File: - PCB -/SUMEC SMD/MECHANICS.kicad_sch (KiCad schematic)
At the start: 9 parts, among them J1 Conn_01x01_Pin, SW1 SW_SPDT, SW3 SW_Push

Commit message: PCB Schematic SMD
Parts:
- SW3: footprint Button_Switch_THT:SW_PUSH_6mm -> Button_Switch_SMD:SW_SPST_B3U-1000P
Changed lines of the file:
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@@
       (effects (font (size 1.27 1.27)))
     )
-    (property "Footprint" "Button_Switch_THT:SW_PUSH_6mm" (at 92.71 125.73 0)
+    (property "Footprint" "Button_Switch_SMD:SW_SPST_B3U-1000P" (at 92.71 125.73 0)
       (effects (font (size 1.27 1.27)) hide)
     )

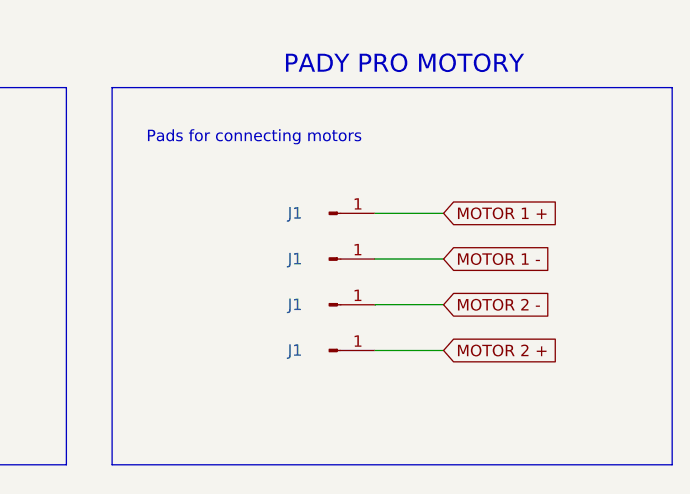
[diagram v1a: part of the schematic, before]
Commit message: PCB SMD update
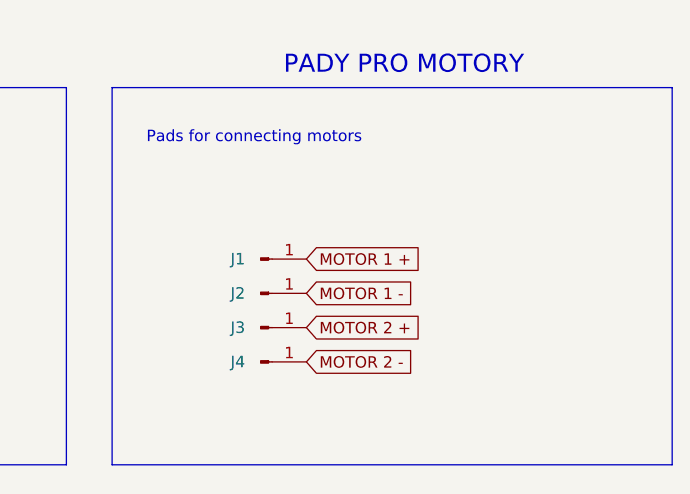
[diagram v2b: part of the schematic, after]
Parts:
- removed J1 (x4): Conn_01x01_Pin, Connector_Wire:SolderWire-0.5sqmm_1x01_D0.9mm_OD2.3mm, symbol Connector:Conn_01x01_Pin
- added J1, J2, J3, J4: Conn_01x01_Pin, Connector_Wire:SolderWire-0.5sqmm_1x01_D0.9mm_OD2.1mm, symbol Connector:Conn_01x01_Pin
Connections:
- net MOTOR 1 +: now also J1.1 (Pin_1)
- net MOTOR 1 -: now also J2.1 (Pin_1)
- net MOTOR 2 +: now also J3.1 (Pin_1)
- net MOTOR 2 -: now also J4.1 (Pin_1)

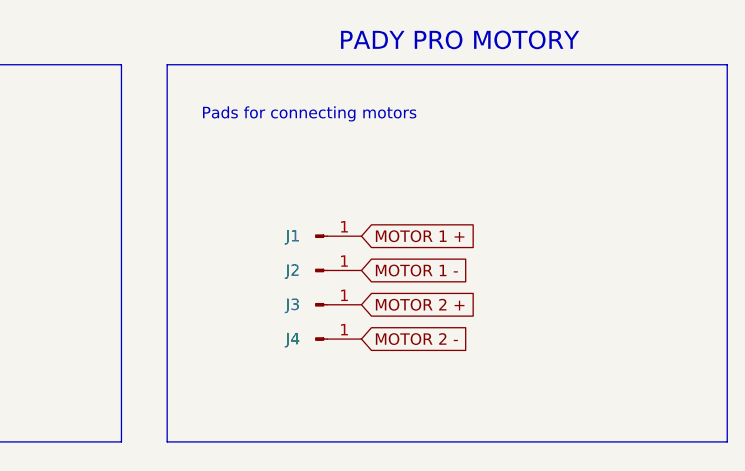
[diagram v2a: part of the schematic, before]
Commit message: PCB smd - schematic update
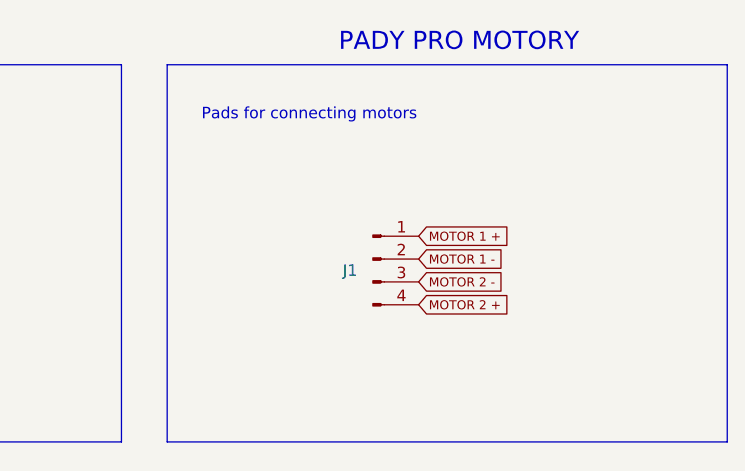
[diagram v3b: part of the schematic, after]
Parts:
- removed J1, J2, J3, J4: Conn_01x01_Pin, Connector_Wire:SolderWire-0.5sqmm_1x01_D0.9mm_OD2.1mm, symbol Connector:Conn_01x01_Pin
- added J1: Conn_01x04_Pin, Connector_PinHeader_2.54mm:PinHeader_1x04_P2.54mm_Vertical, symbol Connector:Conn_01x04_Pin
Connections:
- net MOTOR 1 +: now also J1.1 (Pin_1)
- net MOTOR 1 -: now also J1.2 (Pin_2)
- net MOTOR 2 +: now also J1.4 (Pin_4)
- net MOTOR 2 -: now also J1.3 (Pin_3)
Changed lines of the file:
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@@
     (effects (font (size 1.27 1.27) italic) (justify left bottom))
   )
-  (global_label "MOTOR 1 +" (shape input) (at 170.18 118.11 0) (fields_autoplaced)
-    (effects (font (size 1.27 1.27)) (justify left))
-    (property "Intersheetrefs" "${INTERSHEET_REFS}" (at 184.1529 118.11 0)
-      (effects (font (size 1.27 1.27)) (justify left) hide)
-    )
-  )
-  (global_label "MOTOR 2 +" (shape input) (at 170.18 125.73 0) (fields_autoplaced)
-    (effects (font (size 1.27 1.27)) (justify left))
-    (property "Intersheetrefs" "${INTERSHEET_REFS}" (at 184.1529 125.73 0)
-      (effects (font (size 1.27 1.27)) (justify left) hide)
-    )
-  )
-  (global_label "MOTOR 2 -" (shape input) (at 170.18 129.54 0) (fields_autoplaced)
-    (effects (font (size 1.27 1.27)) (justify left))
-    (property "Intersheetrefs" "${INTERSHEET_REFS}" (at 184.1529 129.54 0)
-      (effects (font (size 1.27 1.27)) (justify left) hide)
-    )
-  )
-  (global_label "MOTOR 1 -" (shape input) (at 170.18 121.92 0) (fields_autoplaced)
-    (effects (font (size 1.27 1.27)) (justify left))
-    (property "Intersheetrefs" "${INTERSHEET_REFS}" (at 184.1529 121.92 0)
+  (global_label "MOTOR 1 +" (shape input) (at 176.53 118.11 0) (fields_autoplaced)
+    (effects (font (size 1 1)) (justify left))
+    (property "Intersheetrefs" "${INTERSHEET_REFS}" (at 187.5322 118.11 0)
+      (effects (font (size 1.27 1.27)) (justify left) hide)
+    )
+  )
+  (global_label "MOTOR 2 +" (shape input) (at 176.53 125.73 0) (fields_autoplaced)
+    (effects (font (size 1 1)) (justify left))
+    (property "Intersheetrefs" "${INTERSHEET_REFS}" (at 187.5322 125.73 0)
+      (effects (font (size 1.27 1.27)) (justify left) hide)
+    )
+  )
+  (global_label "MOTOR 2 -" (shape input) (at 176.53 123.19 0) (fields_autoplaced)
+    (effects (font (size 1 1)) (justify left))
+    (property "Intersheetrefs" "${INTERSHEET_REFS}" (at 187.5322 123.19 0)
+      (effects (font (size 1.27 1.27)) (justify left) hide)
+    )
+  )
+  (global_label "MOTOR 1 -" (shape input) (at 176.53 120.65 0) (fields_autoplaced)
+    (effects (font (size 1 1)) (justify left))
+    (property "Intersheetrefs" "${INTERSHEET_REFS}" (at 187.5322 120.65 0)
       (effects (font (size 1.27 1.27)) (justify left) hide)
     )
@@
     )
   )
-  (symbol (lib_id "Connector:Conn_01x01_Pin") (at 165.1 121.92 0) (unit 1)
-    (in_bom yes) (on_board yes) (dnp no)
-    (property "Reference" "J2" (at 162.56 121.92 0)
-      (effects (font (size 1.27 1.27)))
-    )
-    (property "Value" "Conn_01x01_Pin" (at 165.735 120.65 0)
-      (effects (font (size 1.27 1.27)) hide)
-    )
-    (property "Footprint" "Connector_Wire:SolderWire-0.5sqmm_1x01_D0.9mm_OD2.1mm" (at 165.1 121.92 0)
-      (effects (font (size 1.27 1.27)) hide)
-    )
-    (property "Datasheet" "~" (at 165.1 121.92 0)
-      (effects (font (size 1.27 1.27)) hide)
-    )
-    (pin "1")
-    (instances
-      (project "sumec"
-        (path "/fc70a1a8-ed7c-4a0f-9b1a-f23293528385/05a35bad-c108-46ad-8f95-76319a60a14f"
-          (reference "J2") (unit 1)
-        )
-      )
-    )
-  )
   (symbol (lib_id "Mechanical:MountingHole") (at 72.39 68.58 0) (unit 1)
     (in_bom yes) (on_board yes) (dnp no) (fields_autoplaced)
@@
     )
   )
+  (symbol (lib_id "Connector:Conn_01x04_Pin") (at 171.45 120.65 0) (unit 1)
+    (in_bom yes) (on_board yes) (dnp no)
+    (property "Reference" "J1" (at 168.91 121.92 0)
+      (effects (font (size 1.27 1.27)))
+    )
+    (property "Value" "Conn_01x04_Pin" (at 172.085 116.84 0)
+      (effects (font (size 1.27 1.27)) hide)
+    )
+    (property "Footprint" "Connector_PinHeader_2.54mm:PinHeader_1x04_P2.54mm_Vertical" (at 171.45 120.65 0)
+      (effects (font (size 1.27 1.27)) hide)
+    )
+    (property "Datasheet" "~" (at 171.45 120.65 0)
+      (effects (font (size 1.27 1.27)) hide)
+    )
+    (pin "1")
+    (pin "2")
+    (pin "3")
+    (pin "4")
+    (instances
+      (project "sumec"
+        (path "/fc70a1a8-ed7c-4a0f-9b1a-f23293528385/05a35bad-c108-46ad-8f95-76319a60a14f"
+          (reference "J1") (unit 1)
+        )
+      )
+    )
+  )
   (symbol (lib_id "power:+3V3") (at 86.36 130.81 90) (unit 1)
     (in_bom yes) (on_board yes) (dnp no) (fields_autoplaced)
@@
         (path "/fc70a1a8-ed7c-4a0f-9b1a-f23293528385/05a35bad-c108-46ad-8f95-76319a60a14f"
           (reference "#PWR02") (unit 1)
-        )
-      )
-    )
-  )
-  (symbol (lib_id "Connector:Conn_01x01_Pin") (at 165.1 125.73 0) (unit 1)
-    (in_bom yes) (on_board yes) (dnp no)
-    (property "Reference" "J3" (at 162.56 125.73 0)
-      (effects (font (size 1.27 1.27)))
-    )
-    (property "Value" "Conn_01x01_Pin" (at 165.735 124.46 0)
-      (effects (font (size 1.27 1.27)) hide)
-    )
-    (property "Footprint" "Connector_Wire:SolderWire-0.5sqmm_1x01_D0.9mm_OD2.1mm" (at 165.1 125.73 0)
-      (effects (font (size 1.27 1.27)) hide)
-    )
-    (property "Datasheet" "~" (at 165.1 125.73 0)
-      (effects (font (size 1.27 1.27)) hide)
-    )
-    (pin "1")
-    (instances
-      (project "sumec"
-        (path "/fc70a1a8-ed7c-4a0f-9b1a-f23293528385/05a35bad-c108-46ad-8f95-76319a60a14f"
-          (reference "J3") (unit 1)
         )
       )
@@
         (path "/fc70a1a8-ed7c-4a0f-9b1a-f23293528385/05a35bad-c108-46ad-8f95-76319a60a14f"
           (reference "H1") (unit 1)
-        )
-      )
-    )
-  )
-  (symbol (lib_id "Connector:Conn_01x01_Pin") (at 165.1 118.11 0) (unit 1)
-    (in_bom yes) (on_board yes) (dnp no)
-    (property "Reference" "J1" (at 162.56 118.11 0)
-      (effects (font (size 1.27 1.27)))
-    )
-    (property "Value" "Conn_01x01_Pin" (at 165.735 116.84 0)
-      (effects (font (size 1.27 1.27)) hide)
-    )
-    (property "Footprint" "Connector_Wire:SolderWire-0.5sqmm_1x01_D0.9mm_OD2.1mm" (at 165.1 118.11 0)
-      (effects (font (size 1.27 1.27)) hide)
-    )
-    (property "Datasheet" "~" (at 165.1 118.11 0)
-      (effects (font (size 1.27 1.27)) hide)
-    )
-    (pin "1")
-    (instances
-      (project "sumec"
-        (path "/fc70a1a8-ed7c-4a0f-9b1a-f23293528385/05a35bad-c108-46ad-8f95-76319a60a14f"
-          (reference "J1") (unit 1)
         )
       )
@@
         )
       )
-    )
-  )
-  (symbol (lib_id "Connector:Conn_01x01_Pin") (at 165.1 129.54 0) (unit 1)
-    (in_bom yes) (on_board yes) (dnp no)
-    (property "Reference" "J4" (at 162.56 129.54 0)
-      (effects (font (size 1.27 1.27)))
-    )
-    (property "Value" "Conn_01x01_Pin" (at 165.735 128.27 0)
-      (effects (font (size 1.27 1.27)) hide)
-    )
-    (property "Footprint" "Connector_Wire:SolderWire-0.5sqmm_1x01_D0.9mm_OD2.1mm" (at 165.1 129.54 0)
-      (effects (font (size 1.27 1.27)) hide)
-    )
-    (property "Datasheet" "~" (at 165.1 129.54 0)
-      (effects (font (size 1.27 1.27)) hide)
-    )
-    (pin "1")
-    (instances
-      (project "sumec"
-        (path "/fc70a1a8-ed7c-4a0f-9b1a-f23293528385/05a35bad-c108-46ad-8f95-76319a60a14f"
-          (reference "J4") (unit 1)
-        )
-      )
